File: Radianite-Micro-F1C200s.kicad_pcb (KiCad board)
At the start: 2 copper layers, 60.2 x 27.5 mm, 73 parts, among them J1 USB_C_Receptacle_USB2.0, J2 USB_B_Micro, J3 AudioJack4, J4 Conn_01x04, J5 Micro_SD_Card_Det2, J6 Conn_02x14_Counter_Clockwise, SW1 SW_Push, U1 F1C200s, U2 CH340E, U3 JW5211, U4 JW5211, U5 JW5211, U6 W25Q256JWPIQ, Y1 24MHz

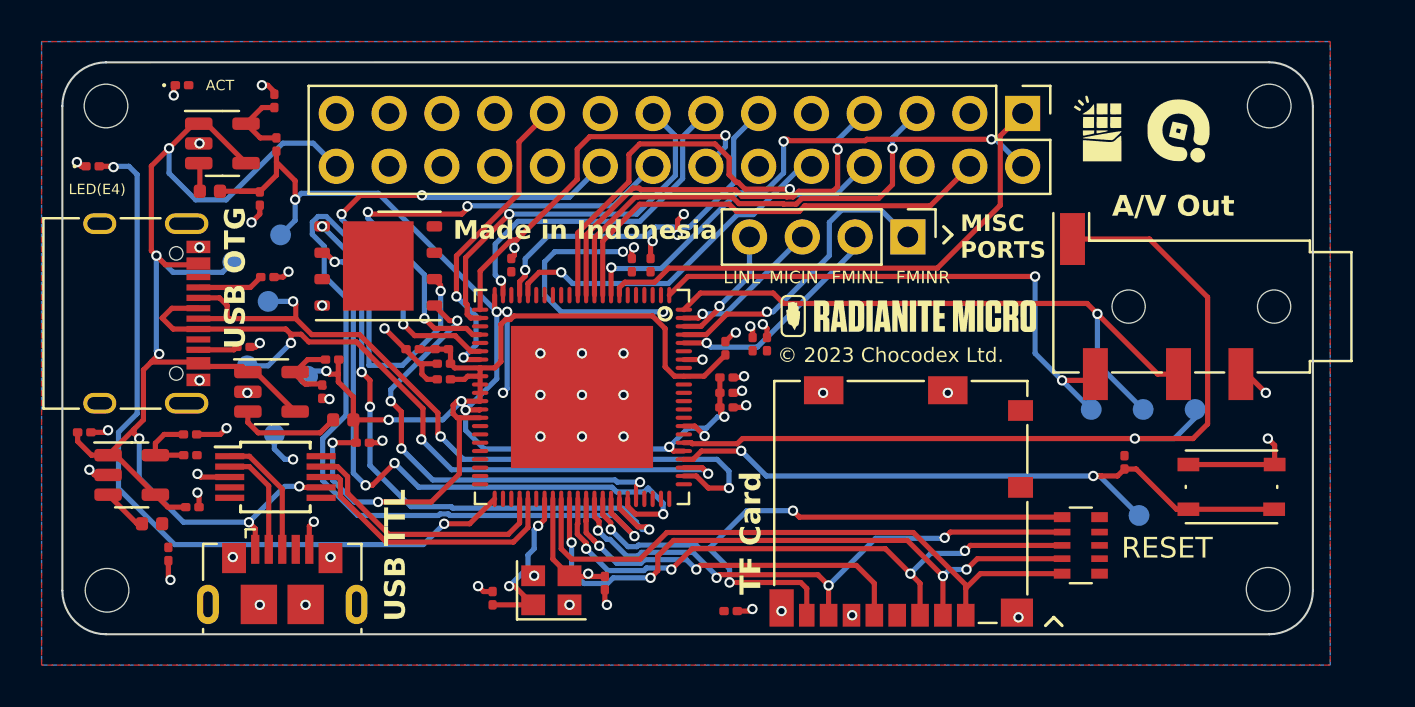
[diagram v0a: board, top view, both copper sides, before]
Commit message: 2.9 change on micro
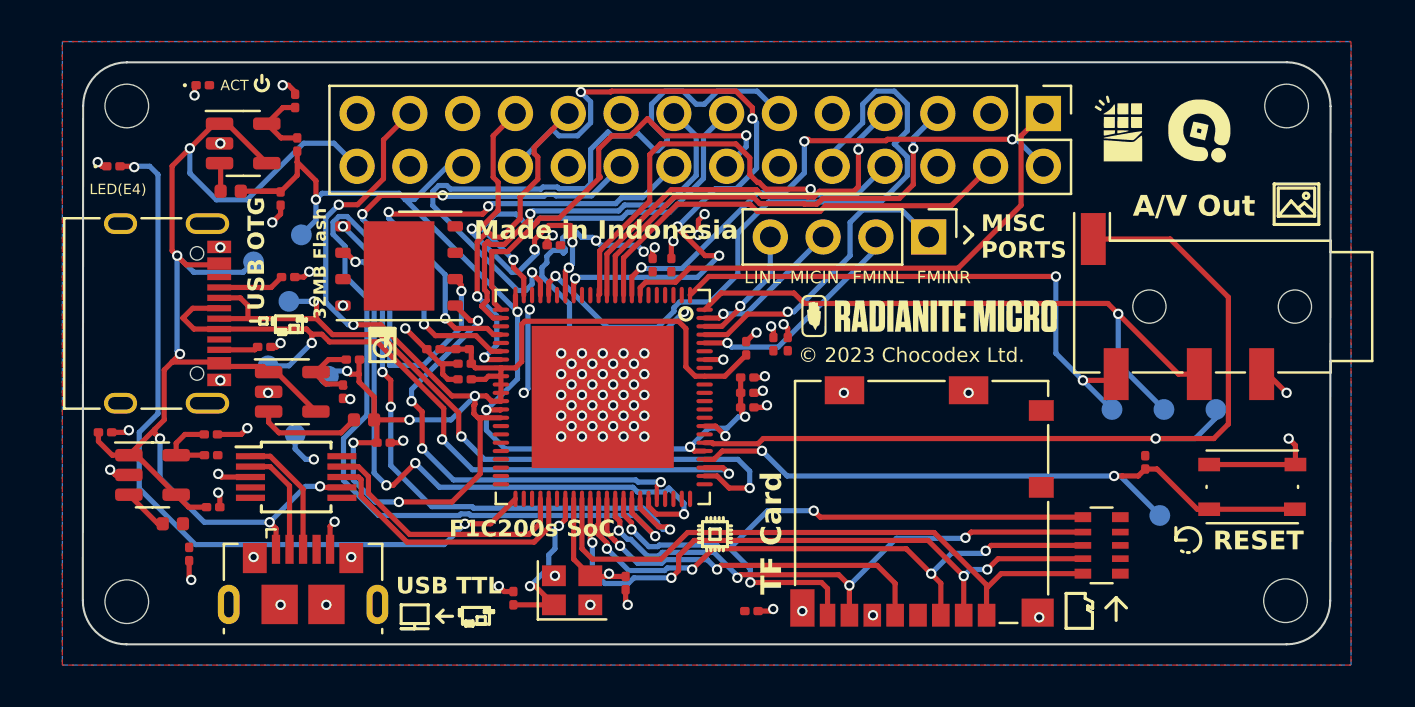
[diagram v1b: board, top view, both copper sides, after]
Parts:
- moved C6 2.26 mm to (123.6, 108.8), turned to 0 degrees
- moved REF** 1.10 mm to (103.1, 125.9)
- moved C1 1.00 mm to (107.3, 121.4)
- moved C10 1.00 mm to (134.2, 113.6)
- moved C11 1.00 mm to (132.9, 113.8)
- moved C12 1.00 mm to (133.0, 115.2)
- moved C13 1.00 mm to (133.0, 115.9)
- moved C14 1.00 mm to (133.0, 116.6)
- moved C15 1.00 mm to (119.4, 115.2)
- moved C16 1.00 mm to (119.4, 114.5)
- moved C17 1.00 mm to (127.1, 125.1)
- moved C18 1.00 mm to (121.7, 125.8)
- moved C19 1.00 mm to (133.2, 126.4)
- moved C2 1.00 mm to (102.1, 117.8)
- moved C3 1.00 mm to (106.1, 123.7)
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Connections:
- J6 pad 21: unconnected-(J6-Pin_21-Pad21) -> /D10
- J6 pad 22: unconnected-(J6-Pin_22-Pad22) -> /D9
- J6 pad 24: unconnected-(J6-Pin_24-Pad24) -> +1V1
- J6 pad 25: unconnected-(J6-Pin_25-Pad25) -> +2V5
- U1 pad 15: unconnected-(U1A-PD9/LCD_D13/DA_LRCK/EINTD9-Pad15) -> /D9
- U1 pad 16: unconnected-(U1A-PD10/LCD_D14/DA_IN/EINTD10-Pad16) -> /D10
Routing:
- net /D9: track 0.00 -> 33.8 mm, vias 0 -> 5
- net +2V5: track 50.8 -> 71.1 mm, vias 5 -> 7
- net /D10: track 0.00 -> 17.6 mm, vias 0 -> 4
- net /D12: track 17.0 -> 33.5 mm
- net /D13: track 17.2 -> 32.9 mm
- net +3V3: track 17.4 -> 22.5 mm, vias 5 -> 6
- net +1V1: track 45.6 -> 49.5 mm
- net /D14: track 16.5 -> 19.7 mm
- net /D15: track 19.1 -> 21.0 mm
- net /D21: track 15.0 -> 16.0 mm
- net /D16: track 18.6 -> 19.5 mm
- net /D4: track 22.4 -> 21.8 mm
- net /D5: track 20.4 -> 19.8 mm
- net GND: track 37.0 -> 37.1 mm, vias 59 -> 91
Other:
- board size 60.2 x 27.5 mm -> 60 x 28 mm
- board text added: "1V1"
- board text added: "2V5"
- board text added: "32MB Flash"
- board text added: "D10"
- board text added: "D9"
- board text added: "F1C200s SoC"
- board text added: "r2.9"
- board text removed: "r2.5"
